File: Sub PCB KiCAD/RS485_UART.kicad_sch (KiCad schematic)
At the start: 7 parts, among them U2 MAX485E

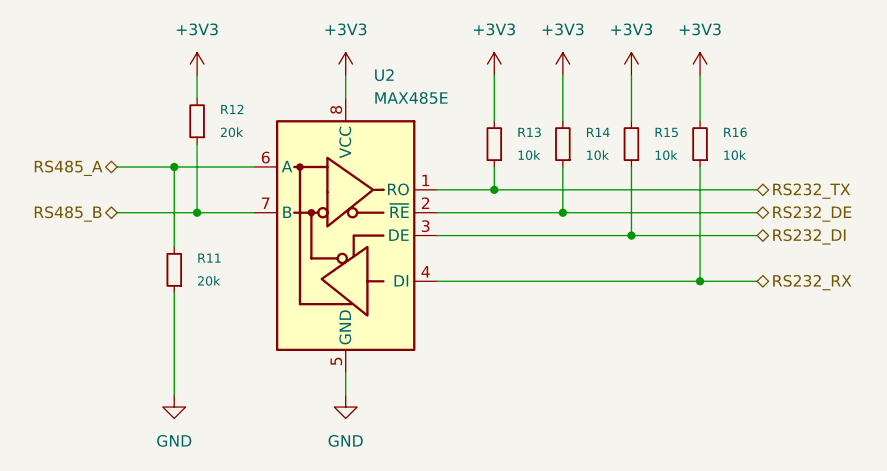
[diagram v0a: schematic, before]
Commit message: .
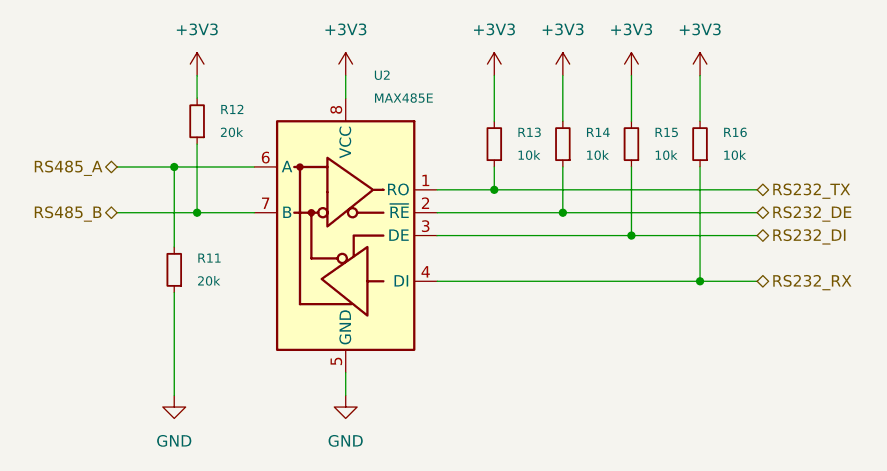
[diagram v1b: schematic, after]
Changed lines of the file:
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@@
 			(effects
 				(font
-					(size 1.27 1.27)
+					(size 1.016 1.016)
 				)
 				(justify right)
@@
 			(effects
 				(font
-					(size 1.27 1.27)
+					(size 1.016 1.016)
 				)
 				(justify right)
